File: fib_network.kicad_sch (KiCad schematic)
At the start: 1 part, among them J3 Bus_M.2_Socket_E

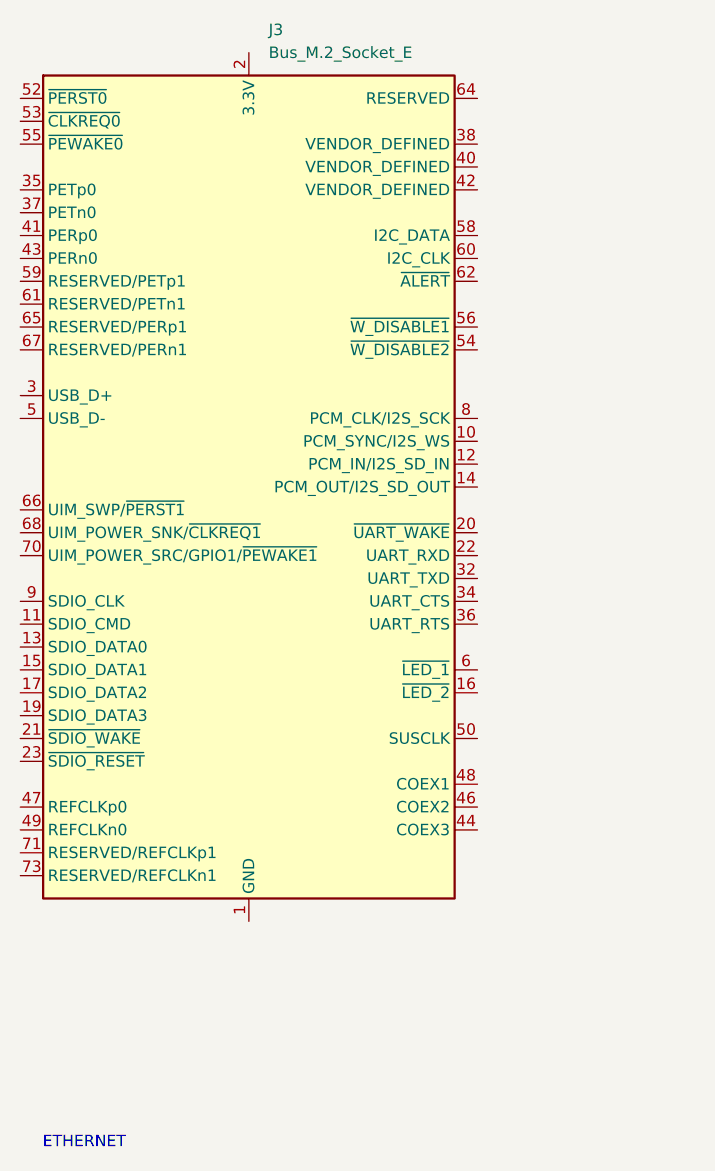
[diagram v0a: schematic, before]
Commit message: added symbol&footprint for orin/sodimm, added a bunch of specs and docs, partially implemented audio, full steam ahead
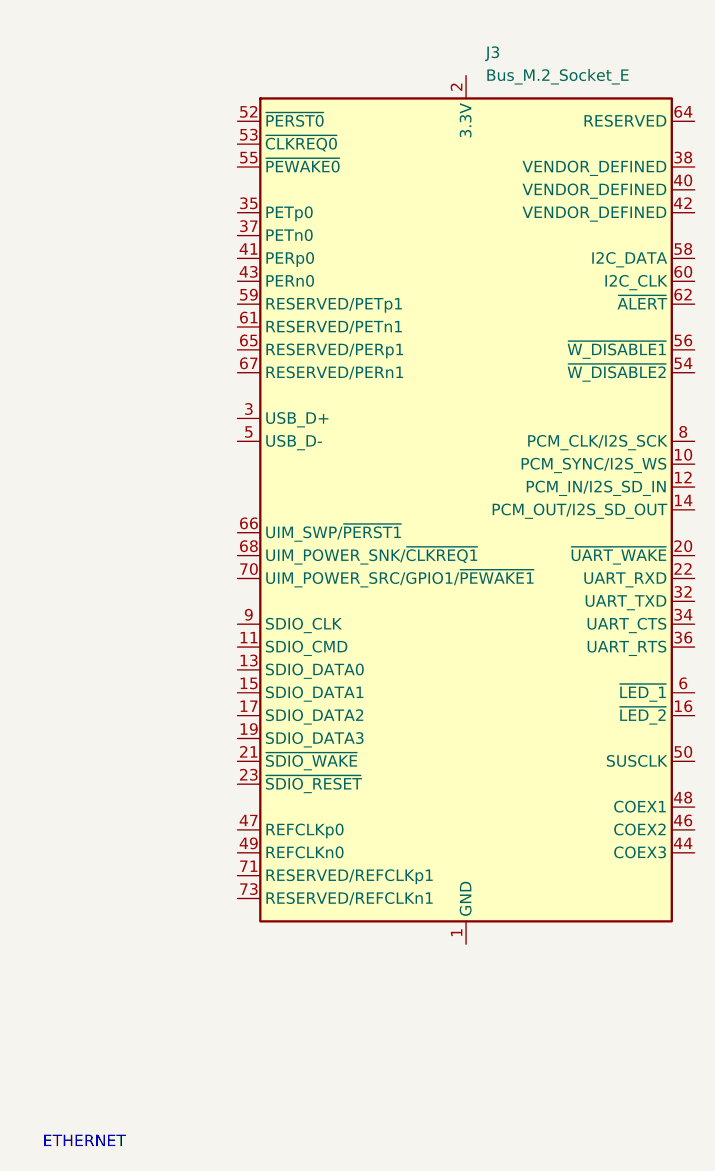
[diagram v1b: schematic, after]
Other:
- moved on the sheet: J3
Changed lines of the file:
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@@
 	(symbol
 		(lib_id "Connector:Bus_M.2_Socket_E")
-		(at 62.23 78.74 0)
+		(at 86.36 81.28 0)
 		(unit 1)
 		(exclude_from_sim no)
@@
 		(fields_autoplaced yes)
 		(property "Reference" "J3"
-			(at 64.4241 27.94 0)
+			(at 88.5541 30.48 0)
 			(effects
 				(font
@@
 		)
 		(property "Value" "Bus_M.2_Socket_E"
-			(at 64.4241 30.48 0)
+			(at 88.5541 33.02 0)
 			(effects
 				(font
@@
 		)
 		(property "Footprint" ""
-			(at 62.23 52.07 0)
+			(at 86.36 54.61 0)
 			(effects
 				(font
@@
 		)
 		(property "Datasheet" "http://read.pudn.com/downloads794/doc/project/3133918/PCIe_M.2_Electromechanical_Spec_Rev1.0_Final_11012013_RS_Clean.pdf#page=150"
-			(at 62.23 52.07 0)
+			(at 86.36 54.61 0)
 			(effects
 				(font
@@
 		)
 		(property "Description" "M.2 Socket 1-SD Mechanical Key E"
-			(at 62.23 78.74 0)
+			(at 86.36 81.28 0)
 			(effects
 				(font
